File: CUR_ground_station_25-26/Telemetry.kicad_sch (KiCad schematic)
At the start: 19 parts, among them J3 Conn_Coaxial_Small, U5 E22-400MM_22S

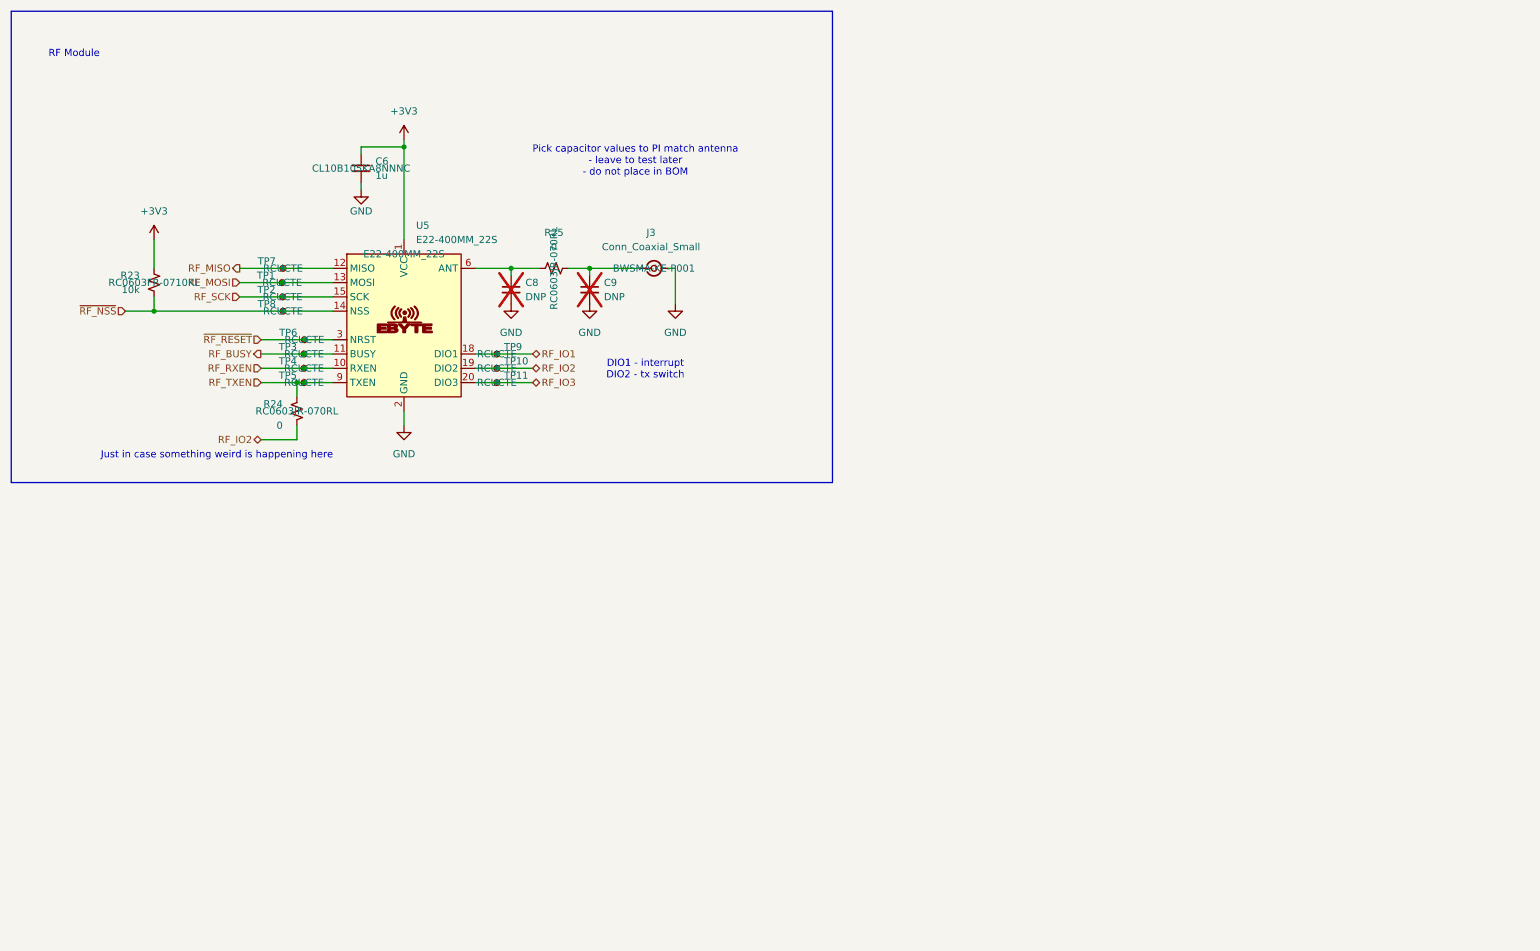
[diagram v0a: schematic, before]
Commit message: changes
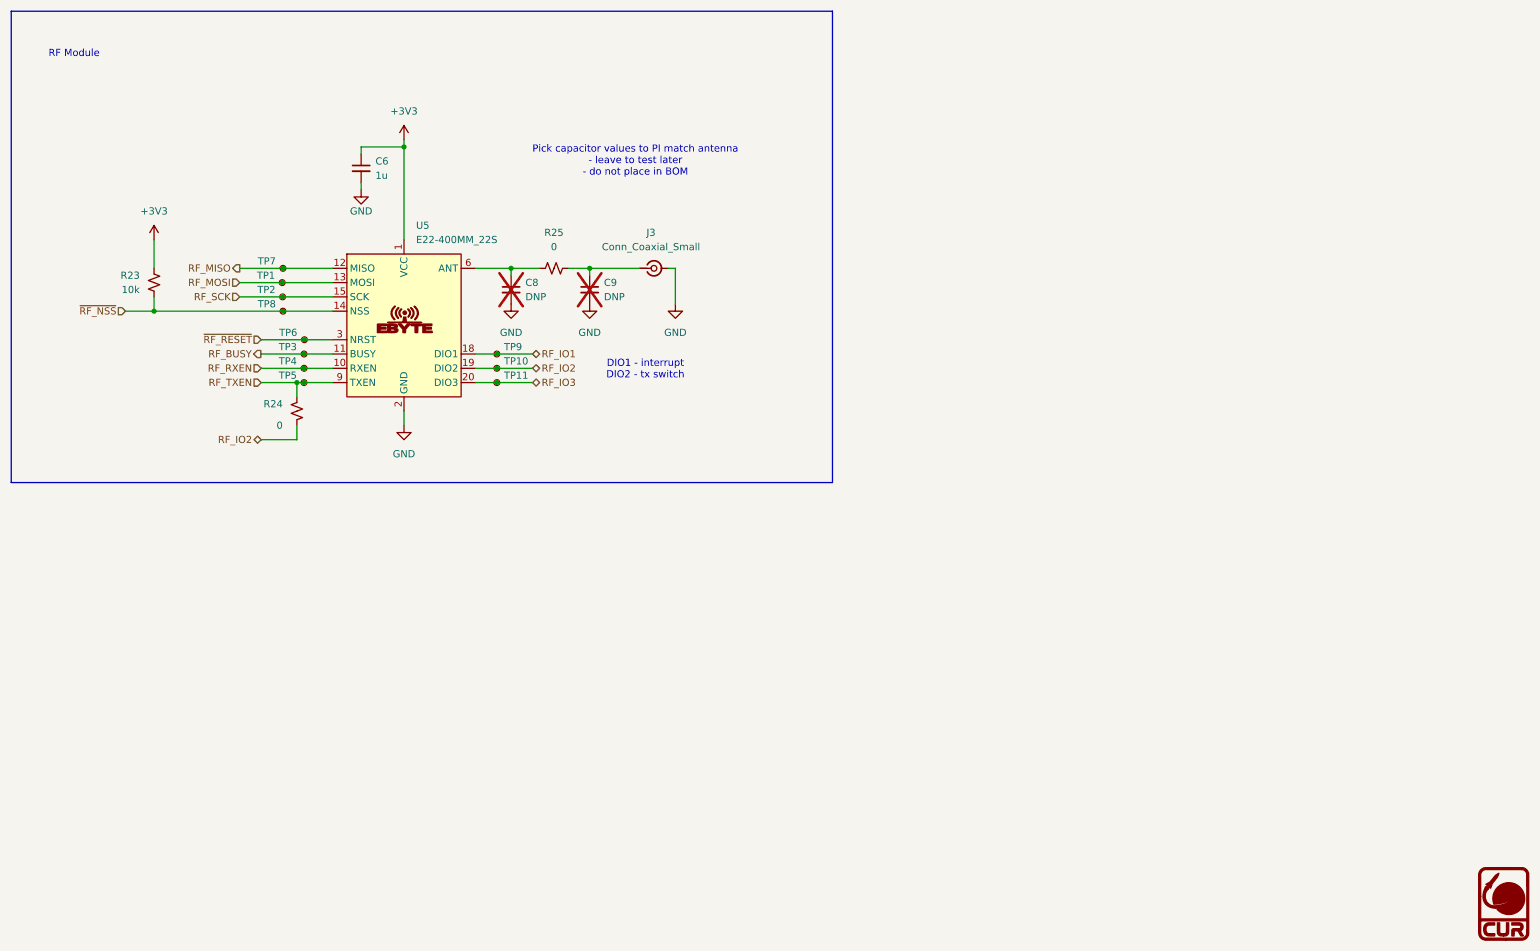
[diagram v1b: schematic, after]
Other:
- note removed: "Just in case something weird is happening here"
- company: (none) -> Clarkson University Rocketry
- title: (none) -> Ground Station
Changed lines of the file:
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@@
 	(generator_version "9.0")
 	(paper "A4")
+	(title_block
+		(title "Ground Station")
+		(date "2026-04-29")
+		(company "Clarkson University Rocketry")
+	)
 	(text "Pick capacitor values to PI match antenna\n- leave to test later\n- do not place in BOM\n"
 		(exclude_from_sim no)
@@
 		(exclude_from_sim no)
 		(at 25.146 22.86 0)
-		(effects
-			(font
-				(size 1.27 1.27)
-			)
-		)
-	)
-	(text "Just in case something weird is happening here"
-		(exclude_from_sim no)
-		(at 50.546 94.234 0)
 		(effects
 			(font
@@
 					(size 1.27 1.27)
 				)
+				(hide yes)
 			)
 		)
@@
 	)
 	(symbol
+		(lib_id "CUR_Logo:LOGO")
+		(at 279.4 173.99 0)
+		(unit 1)
+		(exclude_from_sim no)
+		(in_bom yes)
+		(on_board yes)
+		(dnp no)
+		(fields_autoplaced yes)
+		(property "Reference" "#G3"
+			(at 279.4 167.002 0)
+			(effects
+				(font
+					(size 1.27 1.27)
+				)
+				(hide yes)
+			)
+		)
+		(property "Value" "LOGO"
+			(at 279.4 180.978 0)
+			(effects
+				(font
+					(size 1.27 1.27)
+				)
+				(hide yes)
+			)
+		)
+		(property "Footprint" ""
+			(at 279.4 173.99 0)
+			(effects
+				(font
+					(size 1.27 1.27)
+				)
+				(hide yes)
+			)
+		)
+		(property "Datasheet" ""
+			(at 279.4 173.99 0)
+			(effects
+				(font
+					(size 1.27 1.27)
+				)
+				(hide yes)
+			)
+		)
+		(property "Description" ""
+			(at 279.4 173.99 0)
+			(effects
+				(font
+					(size 1.27 1.27)
+				)
+				(hide yes)
+			)
+		)
+		(instances
+			(project "CUR_ground_station_25-26"
+				(path "/b6f682bd-f29b-4650-adb4-b230be0368ad/b33322ac-e22c-4f1e-acb4-998976370618"
+					(reference "#G3")
+					(unit 1)
+				)
+			)
+		)
+	)
+	(symbol
 		(lib_id "Connector:TestPoint_Small")
 		(at 62.23 66.04 0)
@@
 					(size 1.27 1.27)
 				)
+				(hide yes)
 			)
 		)
@@
 					(size 1.27 1.27)
 				)
+				(hide yes)
 			)
 		)
@@
 					(size 1.27 1.27)
 				)
+				(hide yes)
 			)
 		)
@@
 					(size 1.27 1.27)
 				)
+				(hide yes)
 			)
 		)
@@
 					(size 1.27 1.27)
 				)
+				(hide yes)
 			)
 		)
@@
 					(size 1.27 1.27)
 				)
+				(hide yes)
 			)
 		)
@@
 					(size 1.27 1.27)
 				)
+				(hide yes)
 			)
 		)
@@
 					(size 1.27 1.27)
 				)
+				(hide yes)
 			)
 		)
@@
 					(size 1.27 1.27)
 				)
+				(hide yes)
 			)
 		)
@@
 					(size 1.27 1.27)
 				)
+				(hide yes)
 			)
 		)
@@
 					(size 1.27 1.27)
 				)
+				(hide yes)
 			)
 		)
@@
 					(size 1.27 1.27)
 				)
+				(hide yes)
 			)
 		)
@@
 					(size 1.27 1.27)
 				)
+				(hide yes)
 			)
 		)
@@
 					(size 1.27 1.27)
 				)
+				(hide yes)
 			)
 		)
@@
 					(size 1.27 1.27)
 				)
+				(hide yes)
 			)
 		)
@@
 					(size 1.27 1.27)
 				)
-			)
-		)
+				(hide yes)
+			)
+		)
